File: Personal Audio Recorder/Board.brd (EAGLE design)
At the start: 62.2 x 16.5 mm, 49 parts, among them IC1 MCP1703CB, IC2 MCP73831/OT, J1 PIC_ICSP_MINI_5_PIN, J2 503182-1852, J4 1050170001, U1 XC6204B332MR-SOT23-5

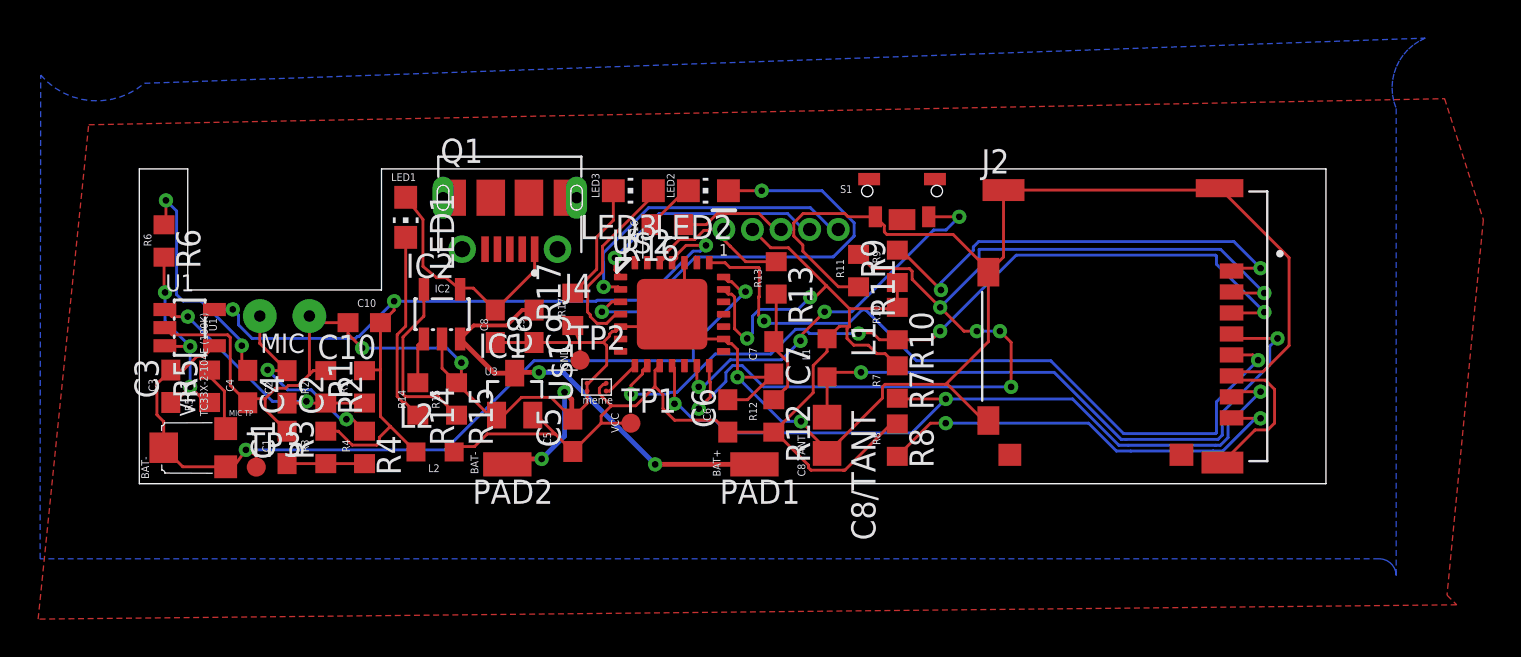
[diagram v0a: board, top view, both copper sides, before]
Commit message: Redid board
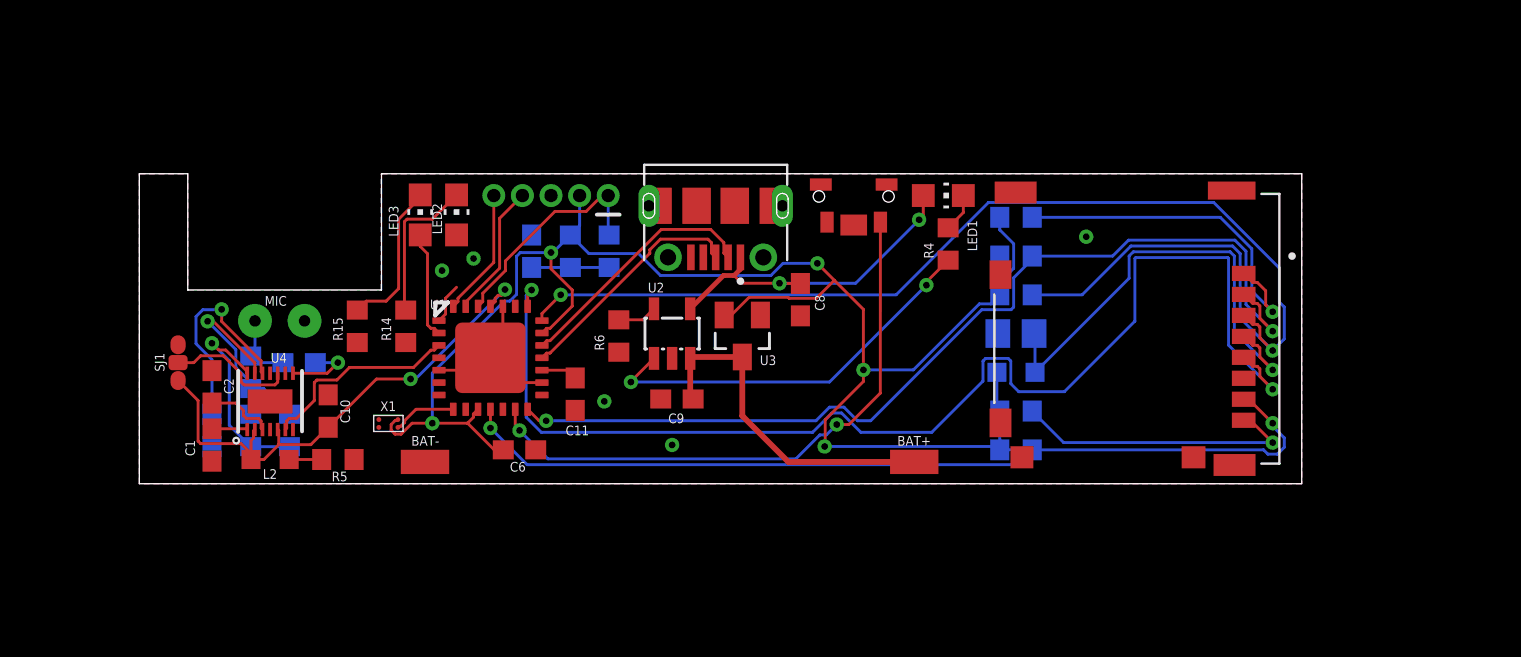
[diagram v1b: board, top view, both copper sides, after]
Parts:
- removed C5: .1uF, rcl:C0603
- removed IC1: MCP1703CB, linear:SOT23
- removed IC2: MCP73831/OT, adafruit:SOT23-5L
- removed J1: PIC_ICSP_MINI_5_PIN, SparkFun-Connectors:PIC_ICSP_MINI_5_PIN
- removed J4: 1050170001, 1050170001:MOLEX_1050170001
- removed PAD1, PAD2: (no value), wirepad:SMD1,27-2,54
- removed Q1: (no value), Extras:9.7ELECTRET
- removed R16, R17: 470, rcl:R0603
- removed TP1, TP2, TP3: TPTP10R, BeagleBone_Blue_R3:TP10R
- removed U$1: SIT1532AC-J5-DCC, Extras:4-UFBGA
- removed U$2: PIC32MX274F256B, Extras:QFN28-ML_6X6MM
- removed VR1: TC33X-2-104E (100K), microbuilder:TRIMPOT_BOURNS_TC33X-2
- added BAT+, BAT-: (no value), wirepad:SMD1,27-2,54
- added C11: 10uF, resistor:C0603
- added CON1: 1050170001, 1050170001:MOLEX_1050170001
- added CON2: PIC_ICSP_MINI_5_PIN, SparkFun-Connectors:PIC_ICSP_MINI_5_PIN
- added MIC: (no value), Extras:9.7ELECTRET
- added SJ1: (no value), Extras:C0R-JMP
- added U2: MCP73831/OT, adafruit:SOT23-5L
- added U3: MCP1703CB, linear:SOT23
- added U4: MAX9814TDFN14, adafruit:TDFN14_3X3MM
- added X1: SIT1532AC-J5-DCC, Extras:4-UFBGA
- C1: value 100pF -> 0.1uF; device rcl:C0603 -> resistor:C0603
- C10: value .1uF -> .01uF; device rcl:C0603 -> resistor:C0603
- C2: value 10pF -> 2.2uF; device rcl:C0603 -> resistor:C0603
- C3: value 100pF -> 0.47uF; device rcl:C0603 -> resistor:C0603
- C4: value 1uF -> 0.1uF; device rcl:C0603 -> resistor:C0603
- C6, C7: value .1uF -> 0.1uF; device rcl:C0603 -> resistor:C0603
- C8, C9: device rcl:C0603 -> resistor:C0603
- R1, R2: value 1M -> 10K; device rcl:R0603 -> resistor:R0603
- R10, R11, R12, R13, R14, R6, R7, R8, R9: device rcl:R0603 -> resistor:R0603
- R15, R4: value 1K -> 470; device rcl:R0603 -> resistor:R0603
- R3: value 1K -> 10K; device rcl:R0603 -> resistor:R0603
- R5: value 10K -> 100; device rcl:R0603 -> resistor:R0603
- U1: value XC6204B332MR-SOT23-5 -> PIC32MX274F256B; device Extras:SOT-23-5 -> Extras:QFN28-ML_6X6MM
- moved R4 32.4 mm to (42.4, 12.6), turned to 90 degrees
- moved LED1 28.2 mm to (42.2, 15.1), turned to 270 degrees
- moved R6 24.4 mm to (25.1, 7.75), turned to 90 degrees
- moved C8 16.1 mm to (34.7, 9.65)
- moved U1 15.9 mm to (18.4, 6.60), turned to 0 degrees
- moved C7 13.9 mm to (20.6, 12.2), flipped to the bottom, turned to 90 degrees
- moved R12 13.7 mm to (22.6, 12.2), flipped to the bottom
- moved LED2 13.3 mm to (16.6, 14.1), turned to 0 degrees
- moved C8/TANT 11.3 mm to (46.0, 7.87), flipped to the bottom, turned to 0 degrees
- moved LED3 11.2 mm to (14.7, 14.1), turned to 0 degrees
- moved C6 11.1 mm to (19.9, 1.78), turned to 0 degrees
- moved L1 9.94 mm to (46.0, 5.84), flipped to the bottom, turned to 180 degrees
- moved R8 9.84 mm to (46.0, 9.91), flipped to the bottom, turned to 0 degrees
- moved R9 9.81 mm to (46.0, 3.81), flipped to the bottom, turned to 0 degrees
- moved R13 8.87 mm to (24.6, 12.2), flipped to the bottom
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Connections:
- removed net LED3: LED3.A, U$2.4
- removed net N$14: J1.4, U$2.1
- removed net N$15: J1.5, U$2.2
- new net D+: CON1.3, U1.18
- new net D-: CON1.2, U1.19
- new net LED1: LED2.A, U1.1
- new net N$16: C3.1, U4.P$12
- new net N$22: L2.2, R5.2
- new net N$23: SJ1.2, U4.P$10
- new net PGC: CON2.5, U1.28
- new net PGD: CON2.4, U1.27
- new net VCAP: C11.1, U1.17
- net AVCC: now also SJ1.1, U1.25, U4.P$2, U4.P$5; no longer R1.2, R3.2, U$2.25, U1.5
- net GND: now also BAT-.1, C11.2, C2.2, C3.2, CON1.5, CON1.SH1, CON1.SH2, CON1.SH3, CON1.SH4, CON1.SH5, CON1.SH6, CON1.SH7, CON1.SH8, CON2.3, MIC.-, R1.2, R11.1, R14.1, R6.1, SJ1.3, U$3.GND@1, U$3.GND@2, U$3.GND@3, U1.16, U1.24, U1.5, U1.EXP, U2.2, U3.1, U4.P$11, U4.P$4, U4.P$7, U4.P$9, U4.P$THERMAL, X1.1, X1.4; no longer C4.2, C5.2, IC1.1, IC2.2, J1.3, J4.5, J4.SH1, J4.SH2, J4.SH3, J4.SH4, J4.SH5, J4.SH6, J4.SH7, J4.SH8, PAD2.1, Q1.-, R11.2, R16.1, R17.1, R2.1, TP2.TP, U$1.1, U$1.4, U$2.16, U$2.24, U$2.5, U$2.EXP, U1.2
- net LED2: now also LED3.A, U1.2; no longer LED2.A, U$2.3
- net MICOUT: now also U1.3, U4.P$6; no longer C3.2, TP3.TP, U$2.21, U1.4, VR1.1, VR1.2
- net MISO: now also R7.1, U1.11; no longer R7.2, U$2.11
- net MMC_SS: now also R11.2, U1.14; no longer R11.1, U$2.14
- net MOSI: now also R8.1, U1.21; no longer R10.2, U$2.9
- net N$1: now also U4.P$1; no longer R3.1, R4.2
- net N$10: now also R4.1, U2.1; no longer IC2.1, R14.1
- net N$11: now also R12.2; no longer R12.1
- net N$12: now also R6.2, U2.5; no longer IC2.5, R15.2
- net N$13: now also CON2.1, U1.26; no longer J1.1, U$2.26
- net N$17: now also BAT+.1, U2.3, U3.3; no longer IC1.3, IC2.3, PAD1.1
- net N$18: now also R14.2; no longer R16.2
- net N$19: now also R15.2; no longer R17.2
- net N$2: now also U4.P$3; no longer Q1.+, R4.1
- net N$21: now also C4.1, U4.P$8; no longer R5.2, VR1.3
- net N$3: now also R3.1, U4.P$13; no longer C2.2, R1.1, U1.1
- net N$4: now also CON1.1, U2.4; no longer IC2.4, J4.1
- net N$5: now also R10.1; no longer R9.2
- net N$6: now also R1.1, R2.1, U4.P$14; no longer C3.1, R5.1, R6.2, U1.3
- net N$7: now also R9.1; no longer R8.2
- net N$8: now also C4.2, MIC.+, R3.2; no longer C4.1, R6.1
- net N$9: now also R4.2; no longer R14.2
- net PB: now also U1.13; no longer U$2.13
- net RTCCCLK: now also U1.8, X1.2; no longer U$1.2, U$2.8
- net SCK: now also U1.22; no longer U$2.22
- net VCC: now also CON2.2, R10.2, R12.1, R5.1, R7.2, R8.2, R9.2, U1.10, U1.20, U3.2, X1.3; no longer C5.1, IC1.2, J1.2, L2.2, R10.1, R12.2, R7.1, R8.1, R9.1, TP1.TP, U$1.3, U$2.10, U$2.20
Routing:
- net GND: track 162.3 -> 9.18 mm, vias 6 -> 5
- net MICOUT: track 45.4 -> 10.7 mm, vias 2 -> 0
- net MOSI: track 41.8 -> 68.1 mm, vias 4 -> 2
- net SCK: track 38.7 -> 64.5 mm
- net VCC: track 67.4 -> 89.2 mm, vias 2 -> 5
- net N$10: track 2.43 -> 21.1 mm, vias 0 -> 2
- net LED2: track 24.1 -> 5.65 mm, vias 2 -> 0
- net AVCC: track 45.1 -> 27.8 mm, vias 3 -> 2
- net N$15: track 16.5 -> 0.00 mm, vias 1 -> 0
- net D-: track 0.00 -> 13.2 mm
- net N$14: track 12.7 -> 0.00 mm, vias 1 -> 0
- net D+: track 0.00 -> 12.5 mm
- net N$16: track 0.00 -> 11.2 mm, vias 0 -> 1
- net PB: track 20.3 -> 31.1 mm, vias 4 -> 2
- net LED3: track 10.0 -> 0.00 mm
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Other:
- board size 62.2 x 16.5 mm -> 61 x 16.3 mm
- board text added: ""In all criminal prosecutions,the accused shall enjoy the right to a speedy and public trial...""
- board text added: "Rev. 1.2"
- board text added: "Self Defenders 2019"
- board text removed: ""...the right of the people to keep and bear Arms, shall not be infringed.""
- board text removed: "1"
- board text removed: "BAT+"
- board text removed: "BAT-"
- board text removed: "C1"
- board text removed: "C10"
- board text removed: "C2"
- board text removed: "C3"
- board text removed: "C4"
- board text removed: "C5"
- board text removed: "C6"
- board text removed: "C7"
- board text removed: "C8"
- board text removed: "C8 TANT"
- board text removed: "C9"
- board text removed: "GND"
- board text removed: "IC2"
- board text removed: "L1"
- board text removed: "L2"
- board text removed: "LED1"
- board text removed: "LED2"
- board text removed: "LED3"
- board text removed: "MIC"
- board text removed: "MIC TP"
- board text removed: "R1"
- board text removed: "R10"
- board text removed: "R11"
- board text removed: "R12"
- board text removed: "R13"
- board text removed: "R14"
- board text removed: "R15"
- board text removed: "R16"
- board text removed: "R17"
- board text removed: "R2"
- board text removed: "R3"
- board text removed: "R4"
- board text removed: "R5"
- board text removed: "R6"
- board text removed: "R7"
- board text removed: "R8"
- board text removed: "R9"
- board text removed: "S1"
- board text removed: "U1"
- board text removed: "U3"
- board text removed: "VCC"
- board text removed: "meme"
